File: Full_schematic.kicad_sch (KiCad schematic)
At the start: 217 parts, among them IC1 XC7A100T-1FTG256C, J1 FFC3B11-40-T, J3 Conn_ST_STDC14, J5 USB_B_Micro, U1 2S7A_0518S1U, U10 MC14511BDG, U11 MAN72A, U12 MC14511BDG, U13 STM32U545VETxQ, U14 MAN72A, U15 MC14511BDG, U16 MAN72A, U17 MC14511BDG, U18 PTS645SM43SMTR92LFS, U19 PTS645SM43SMTR92LFS, U2 IS66WVE4M16EBLL-70BLI, U3 TPS54294PWP, U4 TPS54325PWPR, U5 SN74ALVC245PWR, U6 IS66WVE4M16EBLL-70BLI, U8 SN74ALVC245PWR, U9 MAN72A, Y1 ASCO, Y2 48MHz

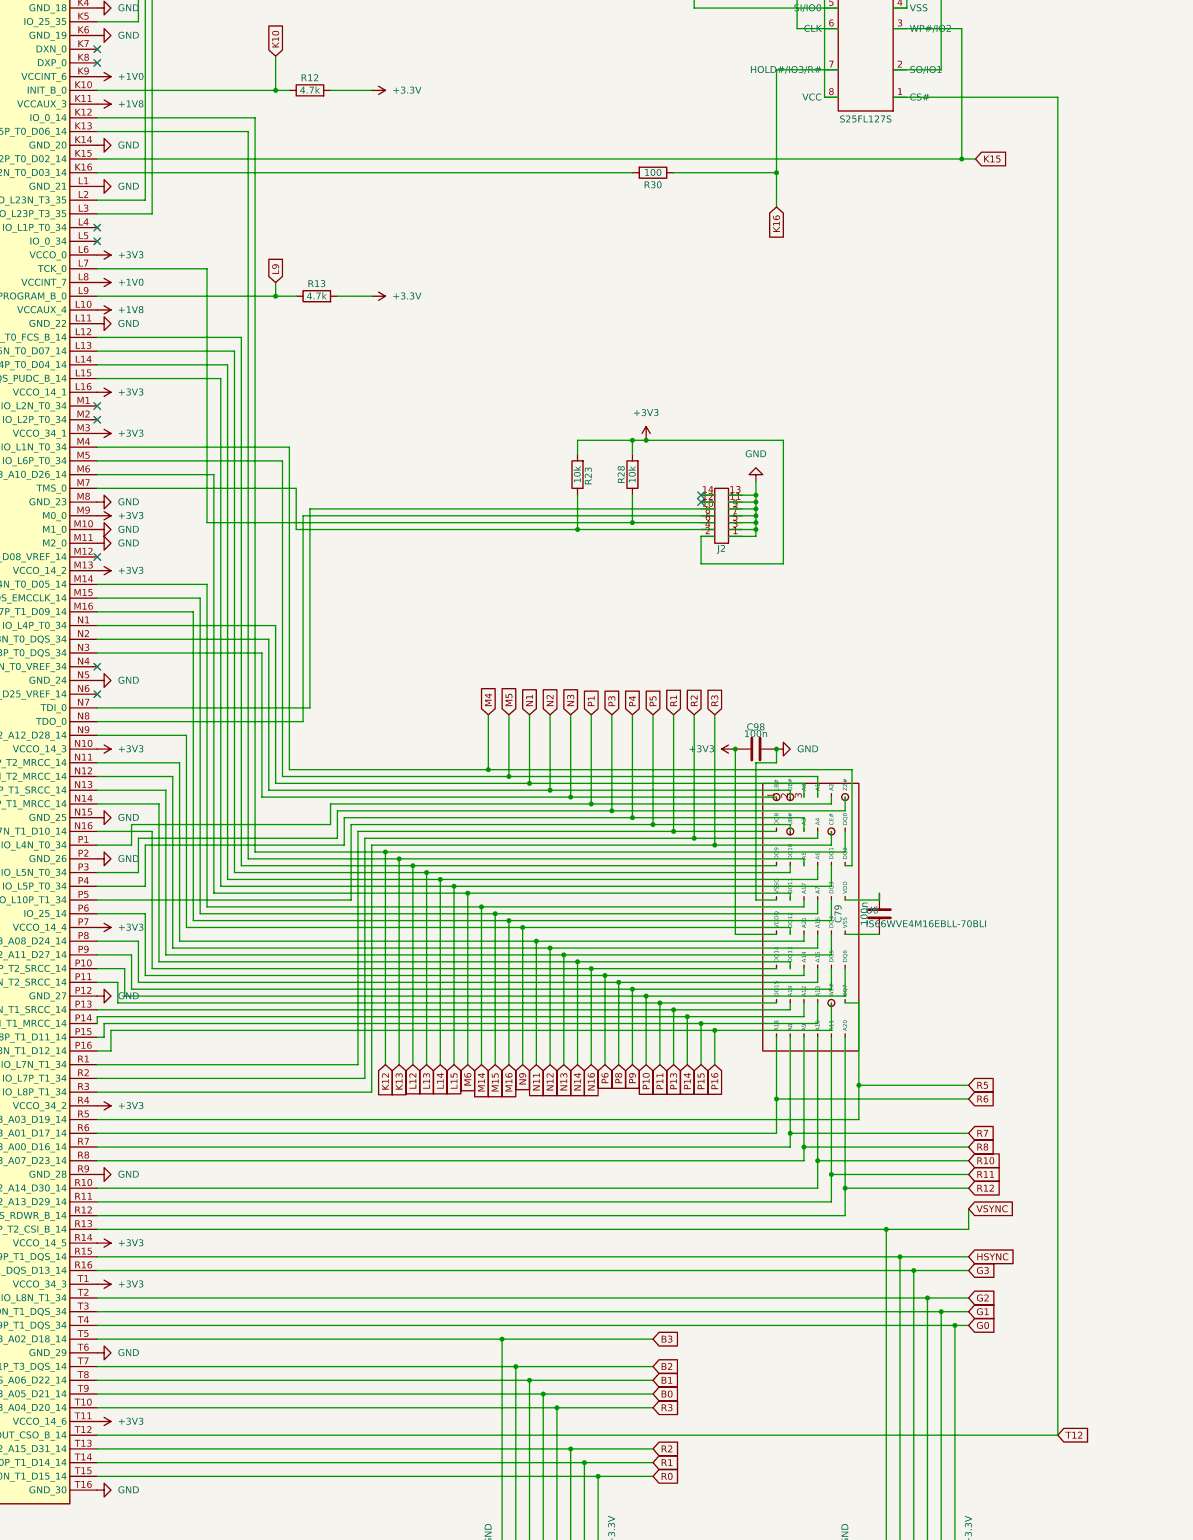
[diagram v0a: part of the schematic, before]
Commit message: commit melding
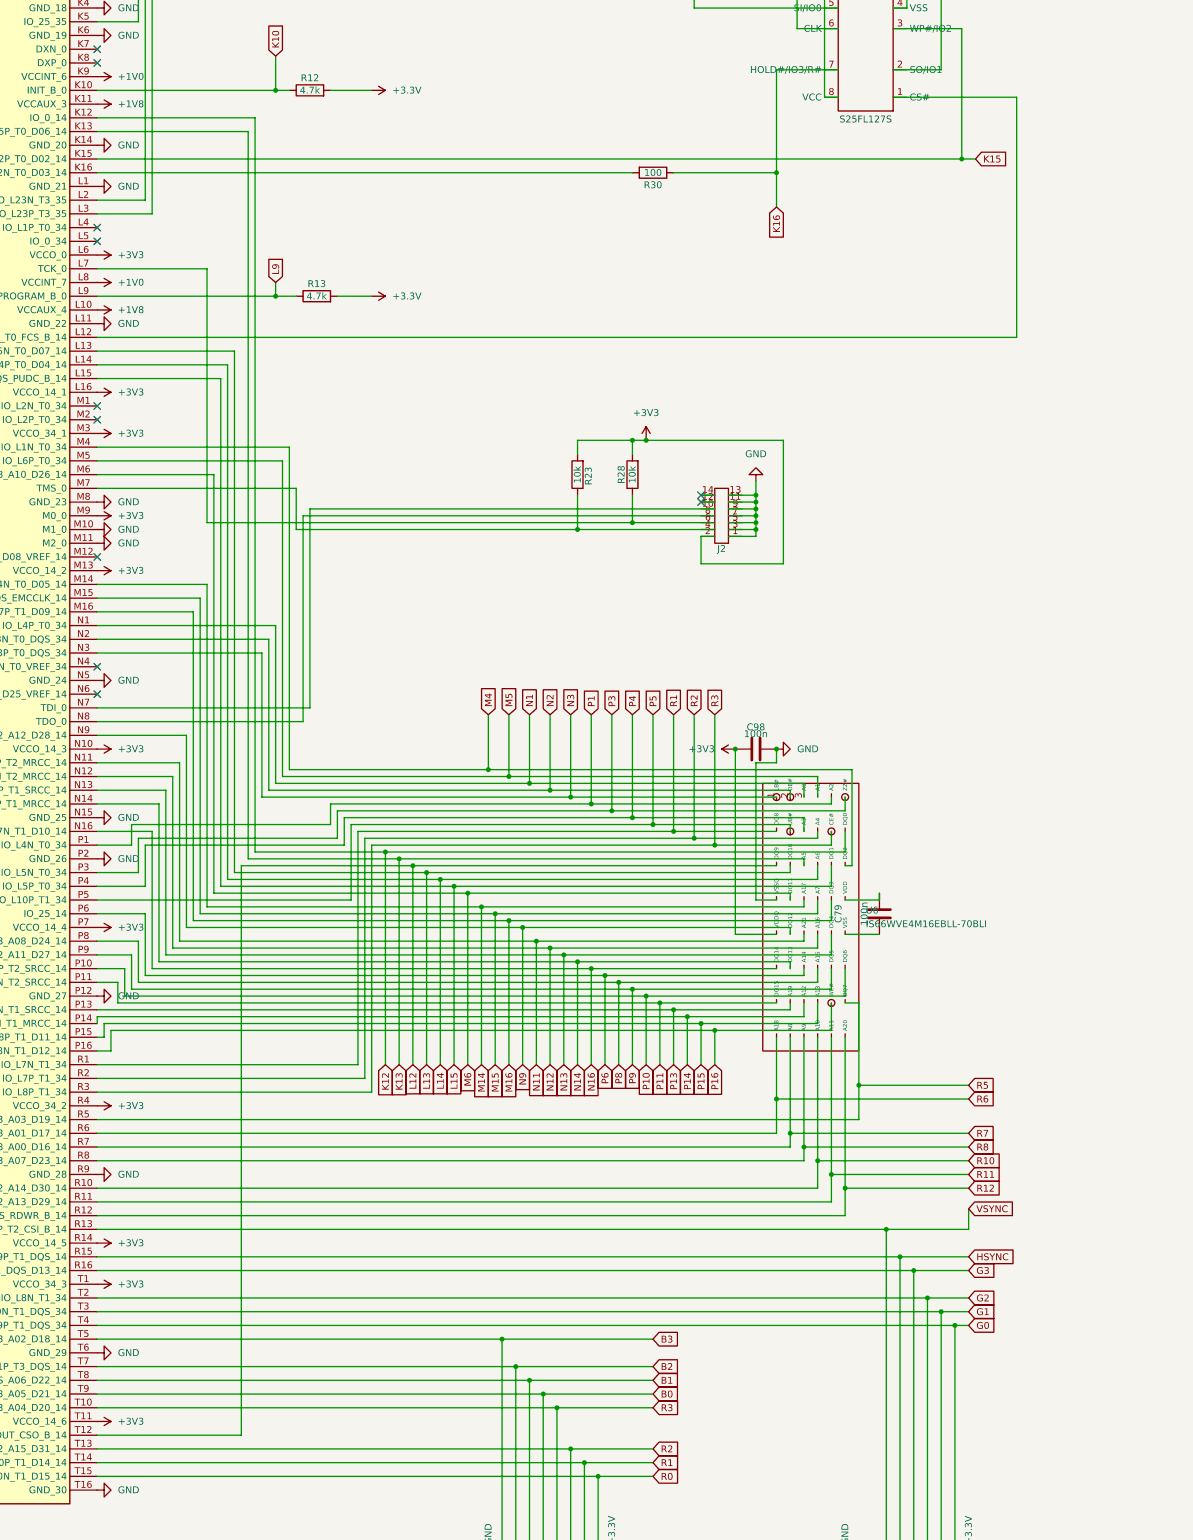
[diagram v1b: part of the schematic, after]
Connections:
- net L12: now also IC1.T12 (IO_L15N_T2_DQS_DOUT_CSO_B_14); no longer IC1.L12 (IO_L6P_T0_FCS_B_14)
- net T12: no longer names the net of U7.1 (CS#)
- net T12: now also IC1.L12 (IO_L6P_T0_FCS_B_14); no longer IC1.T12 (IO_L15N_T2_DQS_DOUT_CSO_B_14)
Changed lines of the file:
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@@
 	(wire
 		(pts
-			(xy 482.6 110.49) (xy 482.6 358.14)
-		)
-		(stroke
-			(width 0)
-			(type default)
-		)
-	)
-	(wire
-		(pts
 			(xy 666.75 588.01) (xy 666.75 675.64)
 		)
@@
 	(wire
 		(pts
+			(xy 474.98 154.94) (xy 474.98 110.49)
+		)
+		(stroke
+			(width 0)
+			(type default)
+		)
+	)
+	(wire
+		(pts
 			(xy 336.55 238.76) (xy 388.62 238.76)
 		)
@@
 	(wire
 		(pts
-			(xy 482.6 110.49) (xy 452.12 110.49)
-		)
-		(stroke
-			(width 0)
-			(type default)
-		)
-	)
-	(wire
-		(pts
 			(xy 450.85 320.04) (xy 450.85 382.27)
 		)
@@
 	(wire
 		(pts
-			(xy 304.8 358.14) (xy 482.6 358.14)
+			(xy 304.8 358.14) (xy 331.47 358.14)
 		)
 		(stroke
@@
 	(wire
 		(pts
-			(xy 331.47 154.94) (xy 331.47 252.73)
-		)
-		(stroke
-			(width 0)
-			(type default)
-		)
-	)
-	(wire
-		(pts
 			(xy 134.62 666.75) (xy 99.06 666.75)
 		)
@@
 	(wire
 		(pts
+			(xy 474.98 110.49) (xy 452.12 110.49)
+		)
+		(stroke
+			(width 0)
+			(type default)
+		)
+	)
+	(wire
+		(pts
 			(xy 120.65 749.3) (xy 191.77 749.3)
 		)
@@
 	(wire
 		(pts
-			(xy 304.8 154.94) (xy 331.47 154.94)
+			(xy 304.8 154.94) (xy 474.98 154.94)
 		)
 		(stroke
@@
 	(wire
 		(pts
+			(xy 331.47 358.14) (xy 331.47 252.73)
+		)
+		(stroke
+			(width 0)
+			(type default)
+		)
+	)
+	(wire
+		(pts
 			(xy 347.98 245.11) (xy 347.98 241.3)
 		)
@@
 				(hide yes)
 			)
-		)
-	)
-	(global_label "T12"
-		(shape input)
-		(at 482.6 358.14 0)
-		(fields_autoplaced yes)
-		(effects
-			(font
-				(size 1.27 1.27)
-			)
-			(justify left)
-		)
-		(property "Intersheetrefs" "${INTERSHEET_REFS}"
-			(at 488.9718 358.14 0)
-			(effects
-				(font
-					(size 1.27 1.27)
-				)
-				(justify left)
-				(hide yes)
-			)
